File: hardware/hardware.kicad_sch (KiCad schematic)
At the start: 8 parts

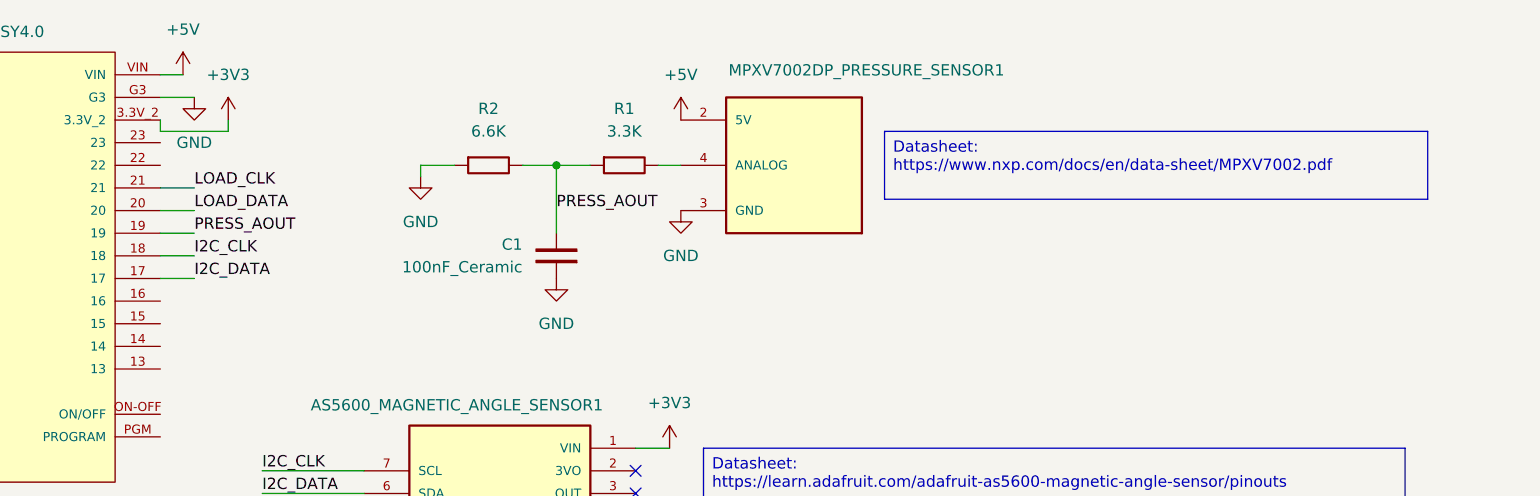
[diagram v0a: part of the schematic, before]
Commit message: won!
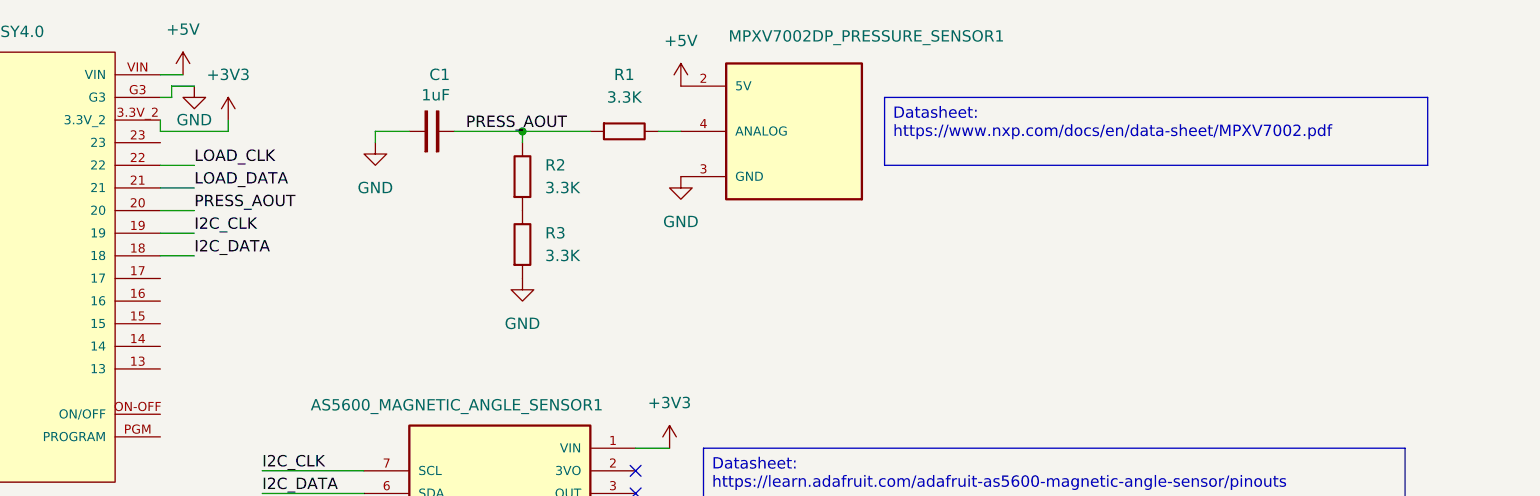
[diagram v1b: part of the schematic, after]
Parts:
- added R3: 3.3K, Resistor_THT:R_Axial_DIN0207_L6.3mm_D2.5mm_P10.16mm_Horizontal, symbol SL_Resistors:10k
- C1: value 100nF_Ceramic -> 1uF
- R2: value 6.6K -> 3.3K
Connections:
- net GND: now also R3.1; no longer R2.1
- net I2C_CLK: now also TEENSY4.0.19; no longer TEENSY4.0.18
- net I2C_DATA: now also TEENSY4.0.18; no longer TEENSY4.0.17
- net LOAD_CLK: now also TEENSY4.0.22; no longer TEENSY4.0.21
- net LOAD_DATA: now also TEENSY4.0.21; no longer TEENSY4.0.20
- net PRESS_AOUT: now also TEENSY4.0.20; no longer TEENSY4.0.19
- new net: R2.1, R3.2
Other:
- moved on the sheet: C1, MPXV7002DP_PRESSURE_SENSOR1, R1, R2
